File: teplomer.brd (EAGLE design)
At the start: 42.9 x 29.2 mm, 5 parts

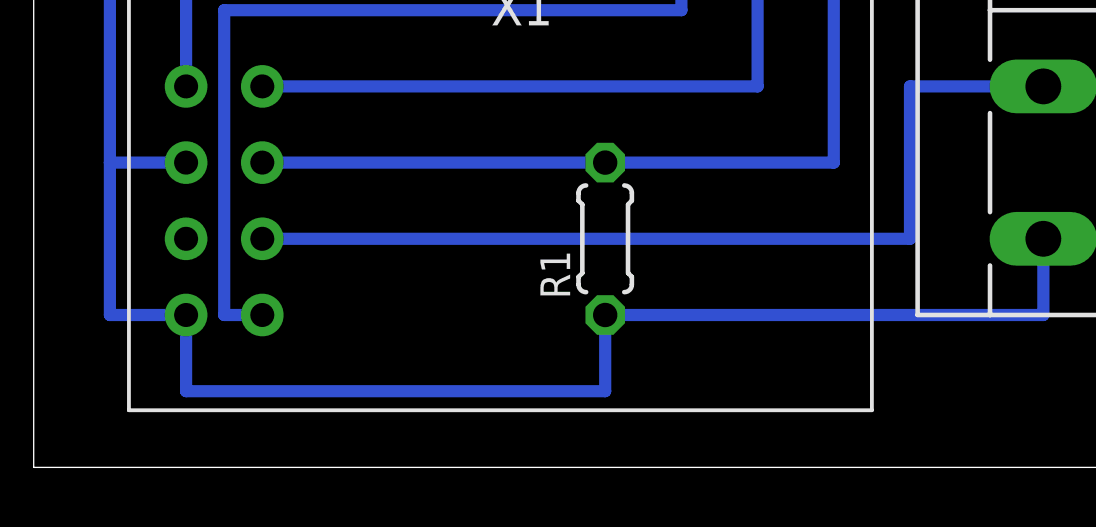
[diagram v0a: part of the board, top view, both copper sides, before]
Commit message: +schenma
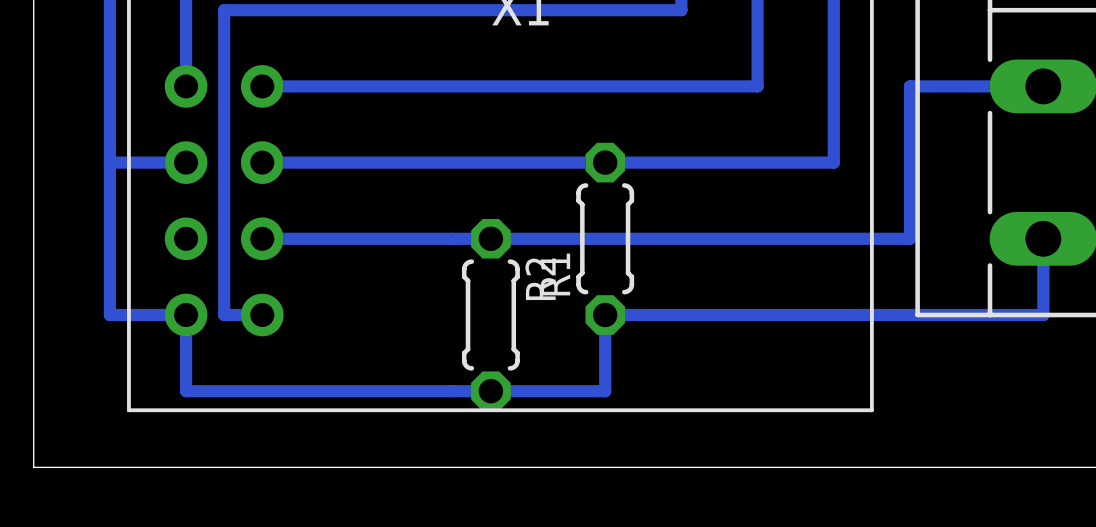
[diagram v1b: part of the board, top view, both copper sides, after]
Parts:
- added R2: 4k7, rcl:0204/5
- R1: value (none) -> 4k7
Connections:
- net +3V3: now also R2.2
- net N$4: now also R2.1
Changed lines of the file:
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@@
 <?xml version="1.0" encoding="utf-8"?>
 <!DOCTYPE eagle SYSTEM "eagle.dtd">
-<eagle version="7.3.0">
+<eagle version="6.5.0">
 <drawing>
 <settings>
@@
 <pass name="Default">
 <param name="RoutingGrid" value="12.5mil"/>
-<param name="AutoGrid" value="1"/>
-<param name="Efforts" value="0"/>
-<param name="TopRouterVariant" value="1"/>
 <param name="tpViaShape" value="round"/>
 <param name="PrefDir.1" value="0"/>
@@
 <param name="PrefDir.14" value="0"/>
 <param name="PrefDir.15" value="0"/>
-<param name="PrefDir.16" value="a"/>
+<param name="PrefDir.16" value="-"/>
 <param name="cfVia" value="8"/>
 <param name="cfNonPref" value="5"/>
@@
 <elements>
 <element name="U$1" library="ESP8266" package="ESP-01" value="ESP8266-01" x="5.08" y="12.7" rot="R270"/>
-<element name="R1" library="rcl" package="0204/5" value="" x="19.05" y="7.62" rot="R90"/>
+<element name="R1" library="rcl" package="0204/5" value="4k7" x="19.05" y="7.62" rot="R90"/>
 <element name="X1" library="con-wago-508" package="W237-3E" value="" x="21.59" y="21.59">
 <attribute name="MPN" value="" x="21.59" y="21.59" size="1.778" layer="27" display="off"/>
@@
 <attribute name="OC_FARNELL" value="unknown" x="34.29" y="15.24" size="1.778" layer="27" rot="R270" display="off"/>
 </element>
+<element name="R2" library="rcl" package="0204/5" value="4k7" x="15.24" y="5.08" rot="R270"/>
 </elements>
 <signals>
@@
 <contactref element="X2" pad="1"/>
 <contactref element="X3" pad="4"/>
-<wire x1="5.08" y1="2.54" x2="19.05" y2="2.54" width="0.4064" layer="16"/>
+<wire x1="5.08" y1="2.54" x2="13.97" y2="2.54" width="0.4064" layer="16"/>
+<wire x1="15.24" y1="2.54" x2="19.05" y2="2.54" width="0.4064" layer="16"/>
 <wire x1="19.05" y1="5.08" x2="19.05" y2="2.54" width="0.4064" layer="16"/>
 <wire x1="19.05" y1="5.08" x2="33.655" y2="5.08" width="0.4064" layer="16"/>
@@
 <wire x1="2.54" y1="21.59" x2="6.35" y2="21.59" width="0.4064" layer="16"/>
 <wire x1="6.35" y1="21.59" x2="6.35" y2="20.955" width="0.4064" layer="16"/>
+<contactref element="R2" pad="2"/>
+<wire x1="15.24" y1="2.54" x2="13.97" y2="2.54" width="0.4064" layer="16"/>
 </signal>
 <signal name="GND">
@@
 <contactref element="X3" pad="3"/>
 <contactref element="U$1" pad="P$6"/>
-<wire x1="7.62" y1="7.62" x2="29.21" y2="7.62" width="0.4064" layer="16"/>
+<wire x1="7.62" y1="7.62" x2="13.97" y2="7.62" width="0.4064" layer="16"/>
+<wire x1="15.24" y1="7.62" x2="29.21" y2="7.62" width="0.4064" layer="16"/>
 <wire x1="29.21" y1="7.62" x2="29.21" y2="12.7" width="0.4064" layer="16"/>
 <wire x1="29.21" y1="12.7" x2="33.655" y2="12.7" width="0.4064" layer="16"/>
+<contactref element="R2" pad="1"/>
+<wire x1="15.24" y1="7.62" x2="13.97" y2="7.62" width="0.4064" layer="16"/>
 </signal>
 </signals>
